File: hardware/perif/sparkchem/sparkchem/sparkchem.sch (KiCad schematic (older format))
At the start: 21 parts

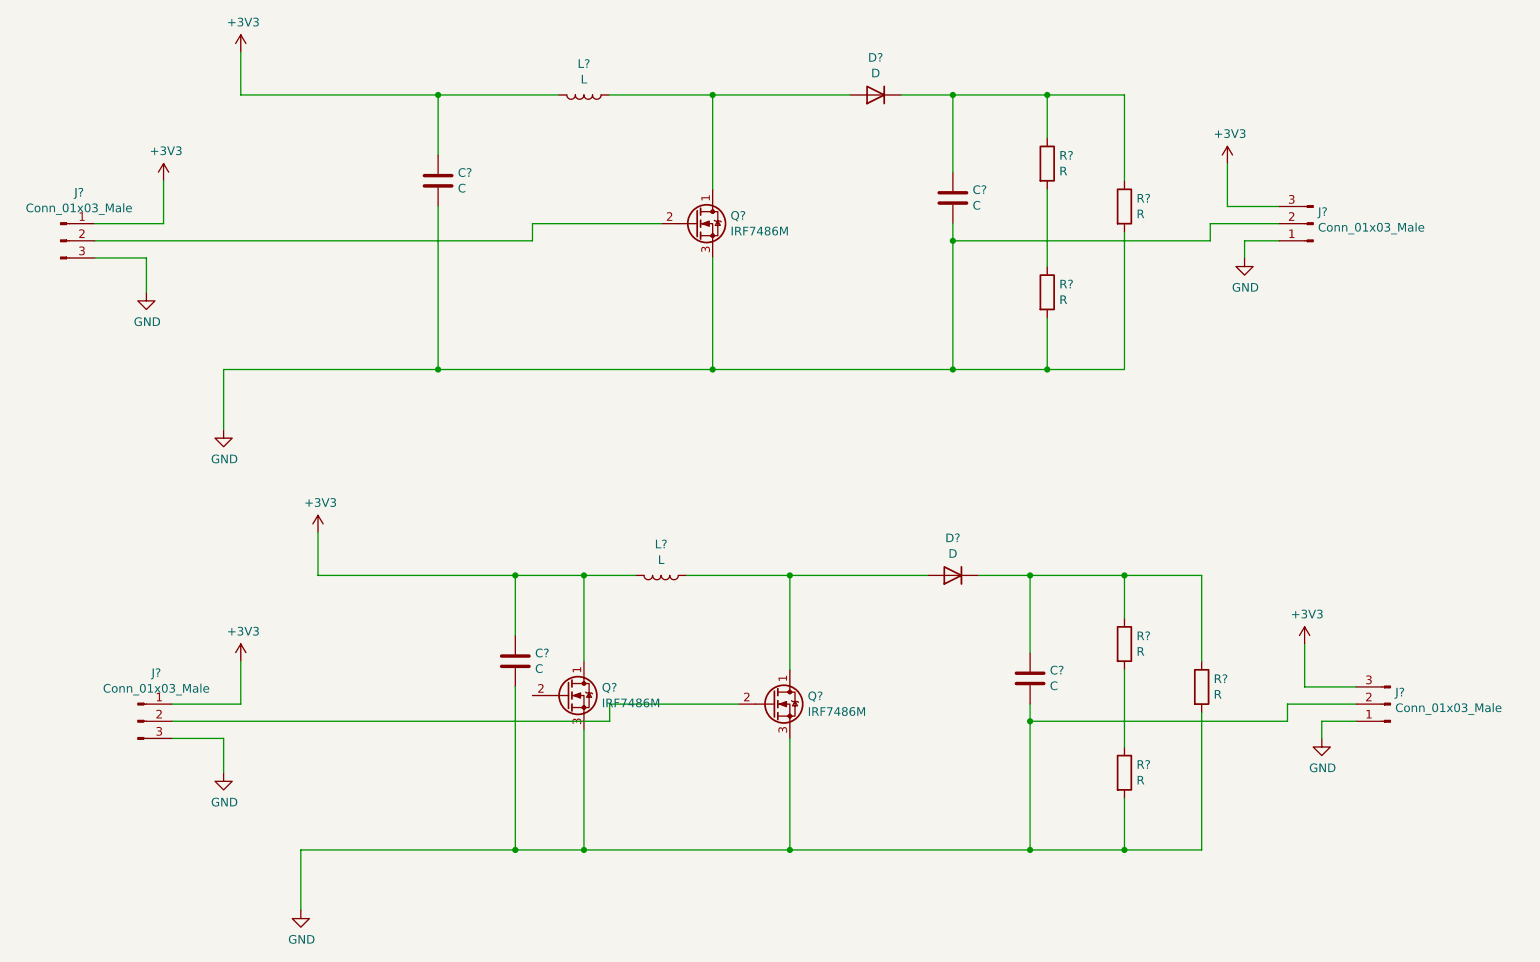
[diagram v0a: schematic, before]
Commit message: periferals
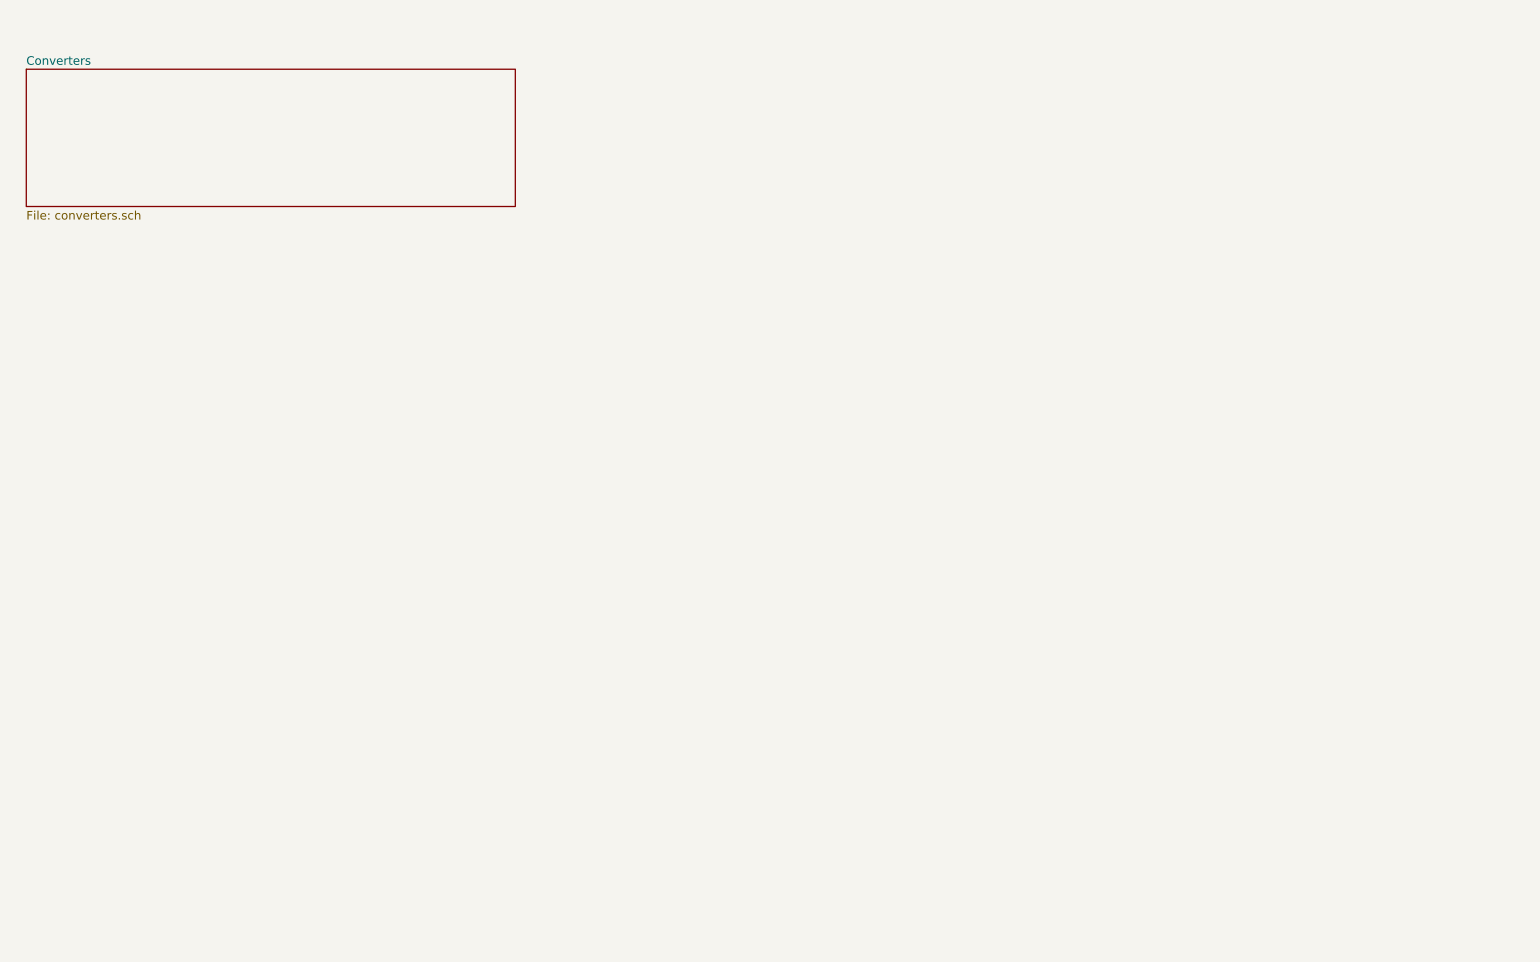
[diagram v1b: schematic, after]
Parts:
- removed C? (x4): C, symbol Device:C
- removed D? (x2): D, symbol Device:D
- removed J? (x4): Conn_01x03_Male, symbol Connector:Conn_01x03_Male
- removed L? (x2): L, symbol Device:L
- removed Q? (x3): IRF7486M, Package_DirectFET:DirectFET_ME, symbol Transistor_FET:IRF7486M
- removed R? (x6): R, symbol Device:R
